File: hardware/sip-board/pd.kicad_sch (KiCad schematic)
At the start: 9 parts, among them U1 TLV75718PDRV, U2 TLV75733PDRV, U3 TLV75710PDRV

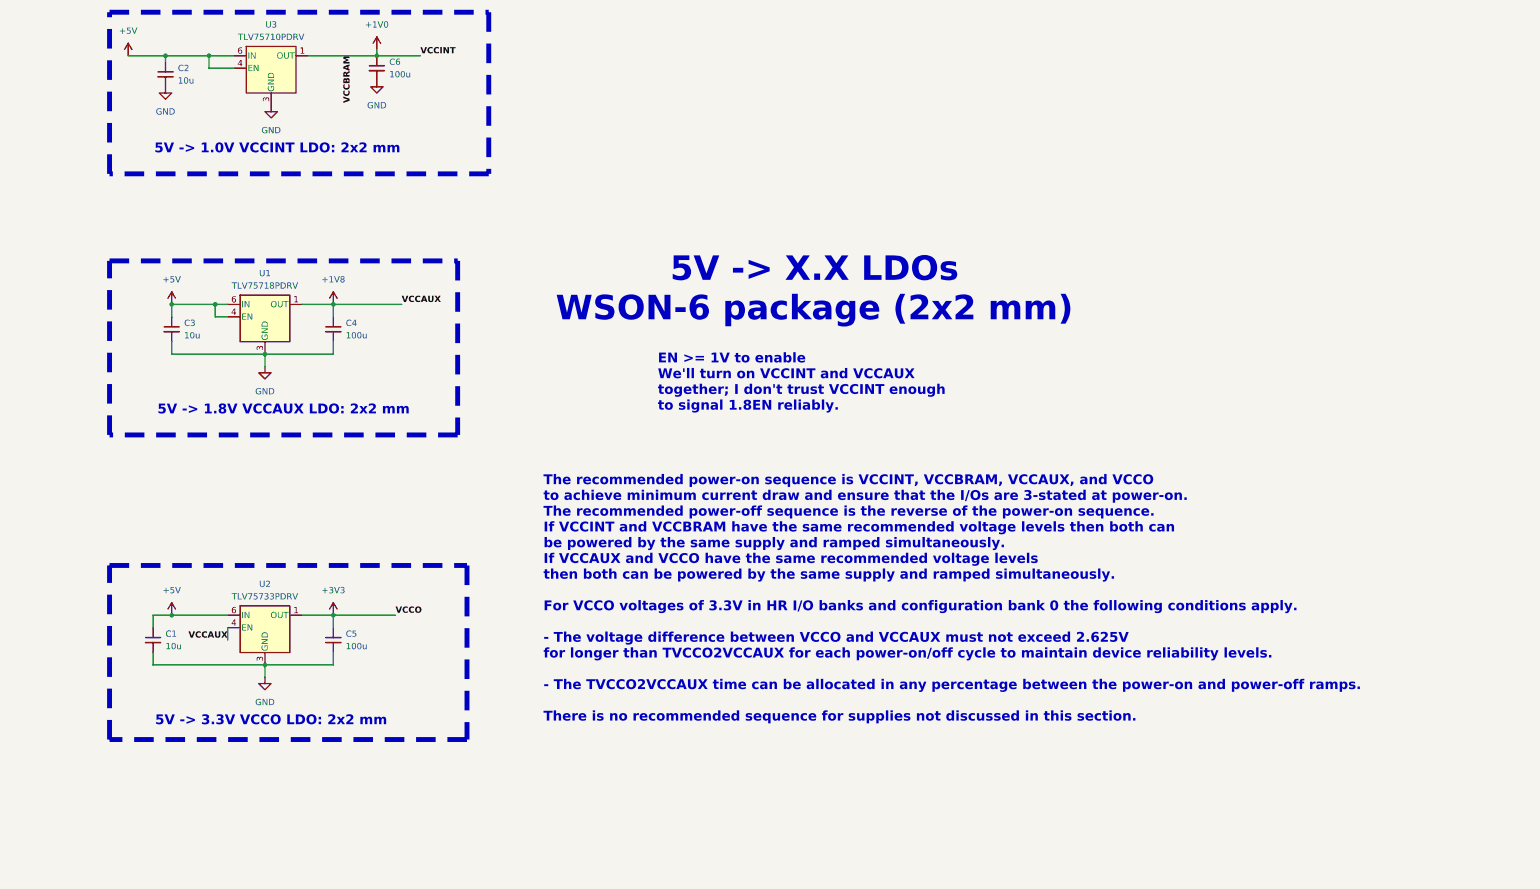
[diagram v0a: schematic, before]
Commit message: raahhhhh my eyeballs hurt
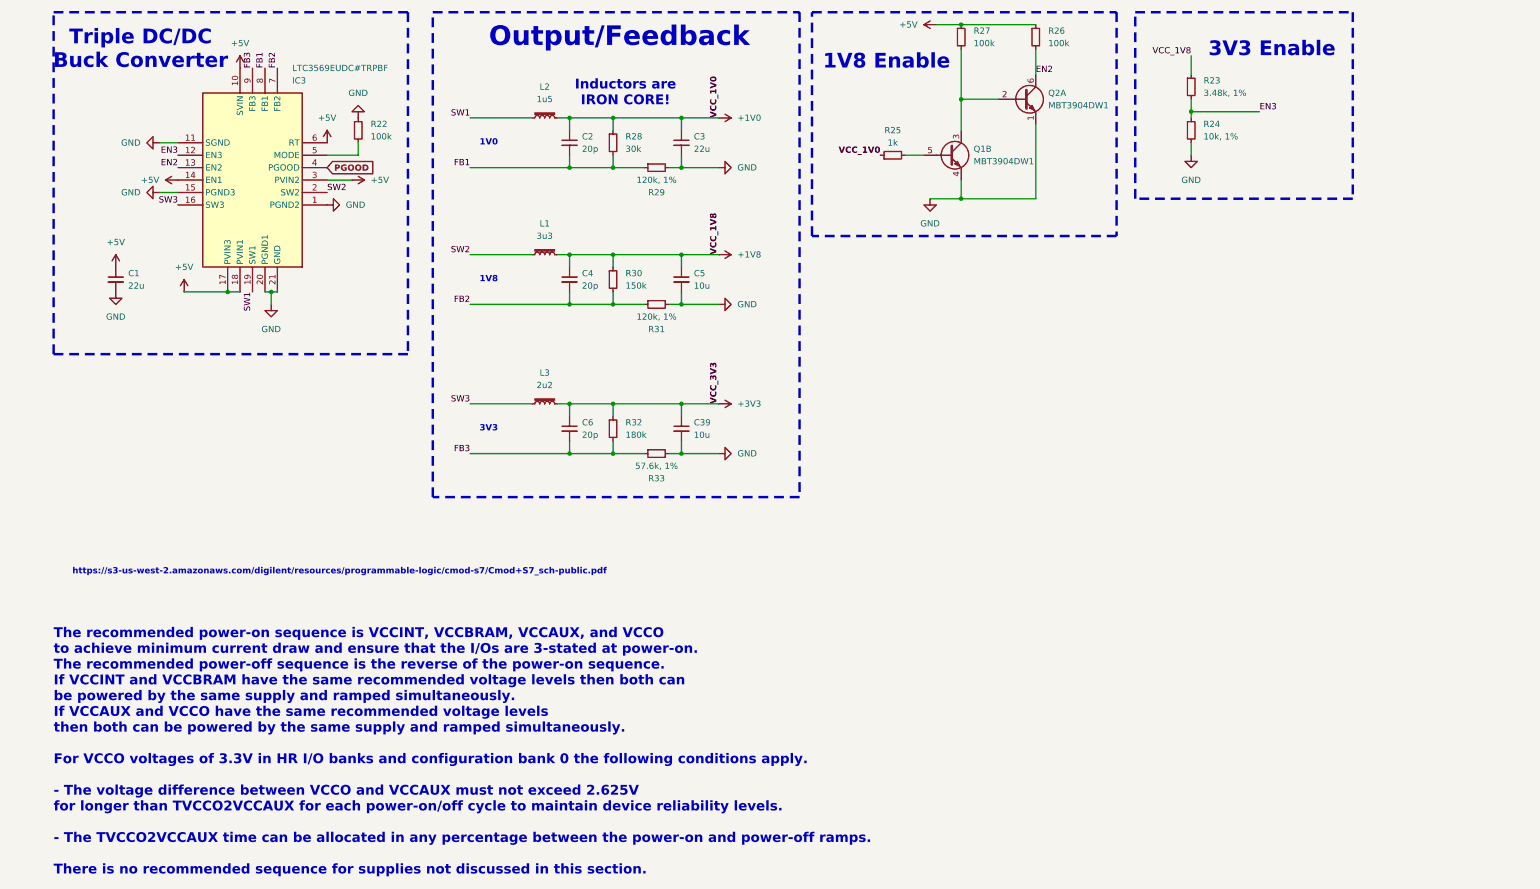
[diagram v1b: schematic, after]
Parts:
- removed U1: TLV75718PDRV, Package_SON:WSON-6-1EP_2x2mm_P0.65mm_EP1x1.6mm, symbol Regulator_Linear:TLV75718PDRV
- removed U2: TLV75733PDRV, Package_SON:WSON-6-1EP_2x2mm_P0.65mm_EP1x1.6mm, symbol Regulator_Linear:TLV75733PDRV
- removed U3: TLV75710PDRV, Package_SON:WSON-6-1EP_2x2mm_P0.65mm_EP1x1.6mm, symbol Regulator_Linear:TLV75710PDRV
- added C39: 10u, Capacitor_SMD:C_0201_0603Metric, symbol Device:C_Small
- added IC3: LTC3569EUDC#TRPBF, hardware:QFN50P300X400X80-21N-D, symbol LTC-3569:LTC3569EUDC#TRPBF
- added L1: 3u3, Capacitor_SMD:C_0201_0603Metric, symbol Device:L_Iron_Small
- added L2: 1u5, Capacitor_SMD:C_0201_0603Metric, symbol Device:L_Iron_Small
- added L3: 2u2, Capacitor_SMD:C_0201_0603Metric, symbol Device:L_Iron_Small
- added Q1, Q2: MBT3904DW1, Package_TO_SOT_SMD:SOT-363_SC-70-6, symbol Transistor_BJT:MBT3904DW1
- added R22, R26, R27: 100k, Resistor_SMD:R_0201_0603Metric, symbol Device:R_Small
- added R23: 3.48k, 1%, Resistor_SMD:R_0201_0603Metric, symbol Device:R_Small
- added R24: 10k, 1%, Resistor_SMD:R_0201_0603Metric, symbol Device:R_Small
- added R25: 1k, Resistor_SMD:R_0201_0603Metric, symbol Device:R_Small
- added R28: 30k, Resistor_SMD:R_0201_0603Metric, symbol Device:R_Small
- added R29, R31: 120k, 1%, Resistor_SMD:R_0201_0603Metric, symbol Device:R_Small
- added R30: 150k, Resistor_SMD:R_0201_0603Metric, symbol Device:R_Small
- added R32: 180k, Resistor_SMD:R_0201_0603Metric, symbol Device:R_Small
- added R33: 57.6k, 1%, Resistor_SMD:R_0201_0603Metric, symbol Device:R_Small
- C1, C3: value 10u -> 22u; footprint Capacitor_SMD:C_0402_1005Metric -> Capacitor_SMD:C_0201_0603Metric
- C2: value 10u -> 20p; footprint Capacitor_SMD:C_0402_1005Metric -> Capacitor_SMD:C_0201_0603Metric
- C4, C6: value 100u -> 20p
- C5: value 100u -> 10u
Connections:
- net +1V0: now also C2.1, C3.1, L2.2, R25.1, R28.1; no longer C6.1
- net +1V8: now also C5.1, L1.2, R23.1, R30.1
- net +3V3: now also C6.1, C39.1, L3.2, R32.1; no longer C5.1
- net +5V: now also IC3.10 (SVIN), IC3.14 (EN1), IC3.17 (PVIN3), IC3.18 (PVIN1), IC3.3 (PVIN2), IC3.6 (RT), R26.1, R27.1; no longer C2.1, C3.1
- net GND: now also C39.2, IC3.1 (PGND2), IC3.11 (SGND), IC3.15 (PGND3), IC3.20 (PGND1), IC3.21 (GND), Q1.4 (E2), Q2.1 (E1), R22.1, R24.2, R29.2, R31.2, R33.2; no longer C2.2, C4.2, C6.2
- new net: IC3.5 (MODE), R22.2
- new net: Q1.3 (C2), Q2.2 (B1), R27.2
- new net: Q1.5 (B2), R25.2
- new net EN2: IC3.13 (EN2), Q2.6 (C1), R26.2
- new net EN3: IC3.12 (EN3), R23.2, R24.1
- new net FB1: C2.2, IC3.8 (FB1), R28.2, R29.1
- new net FB2: C4.2, IC3.7 (FB2), R30.2, R31.1
- new net FB3: C6.2, IC3.9 (FB3), R32.2, R33.1
- new net PGOOD: IC3.4 (PGOOD)
- new net SW1: IC3.19 (SW1), L2.1
- new net SW2: IC3.2 (SW2), L1.1
- new net SW3: IC3.16 (SW3), L3.1
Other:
- note added: "1V0"
- note added: "1V8"
- note added: "1V8 Enable"
- note added: "3V3"
- note added: "3V3 Enable"
- note added: "Inductors are IRON CORE!"
- note added: "Output/Feedback"
- note added: "Triple DC/DC Buck Converter"
- note added: "https://s3-us-west-2.amazonaws.com/digilent/resources/programmable-logic/cmod-s7/Cmod+S7_sch-public.pdf"
- note removed: "5V -> 1.0V VCCINT LDO: 2x2 mm"
- note removed: "5V -> 1.8V VCCAUX LDO: 2x2 mm"
- note removed: "5V -> 3.3V VCCO LDO: 2x2 mm"
- note removed: "5V -> X.X LDOs WSON-6 package (2x2 mm)"
- note removed: "EN >= 1V to enable We'll turn on VCCINT and VCCAUX together; I don't trust VCCINT enough to signal 1.8EN reliably."

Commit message: WE REDOIN PCB
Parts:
- IC3: MPN (none) -> LTC3569EUDC#TRPBF; Manufacturer_Part_Number LTC3569EUDC#TRPBF -> (none)
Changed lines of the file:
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@@
 			)
 		)
-		(property "Manufacturer_Part_Number" "LTC3569EUDC#TRPBF"
+		(property "MPN" "LTC3569EUDC#TRPBF"
 			(at 43.18 -726.34 0)
 			(effects
